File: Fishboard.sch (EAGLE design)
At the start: 21 parts, among them J3 B1, J4 B2, J5 B3, J7 B4, Q1 TIP120, Q2 TIP120, Q3 TIP120

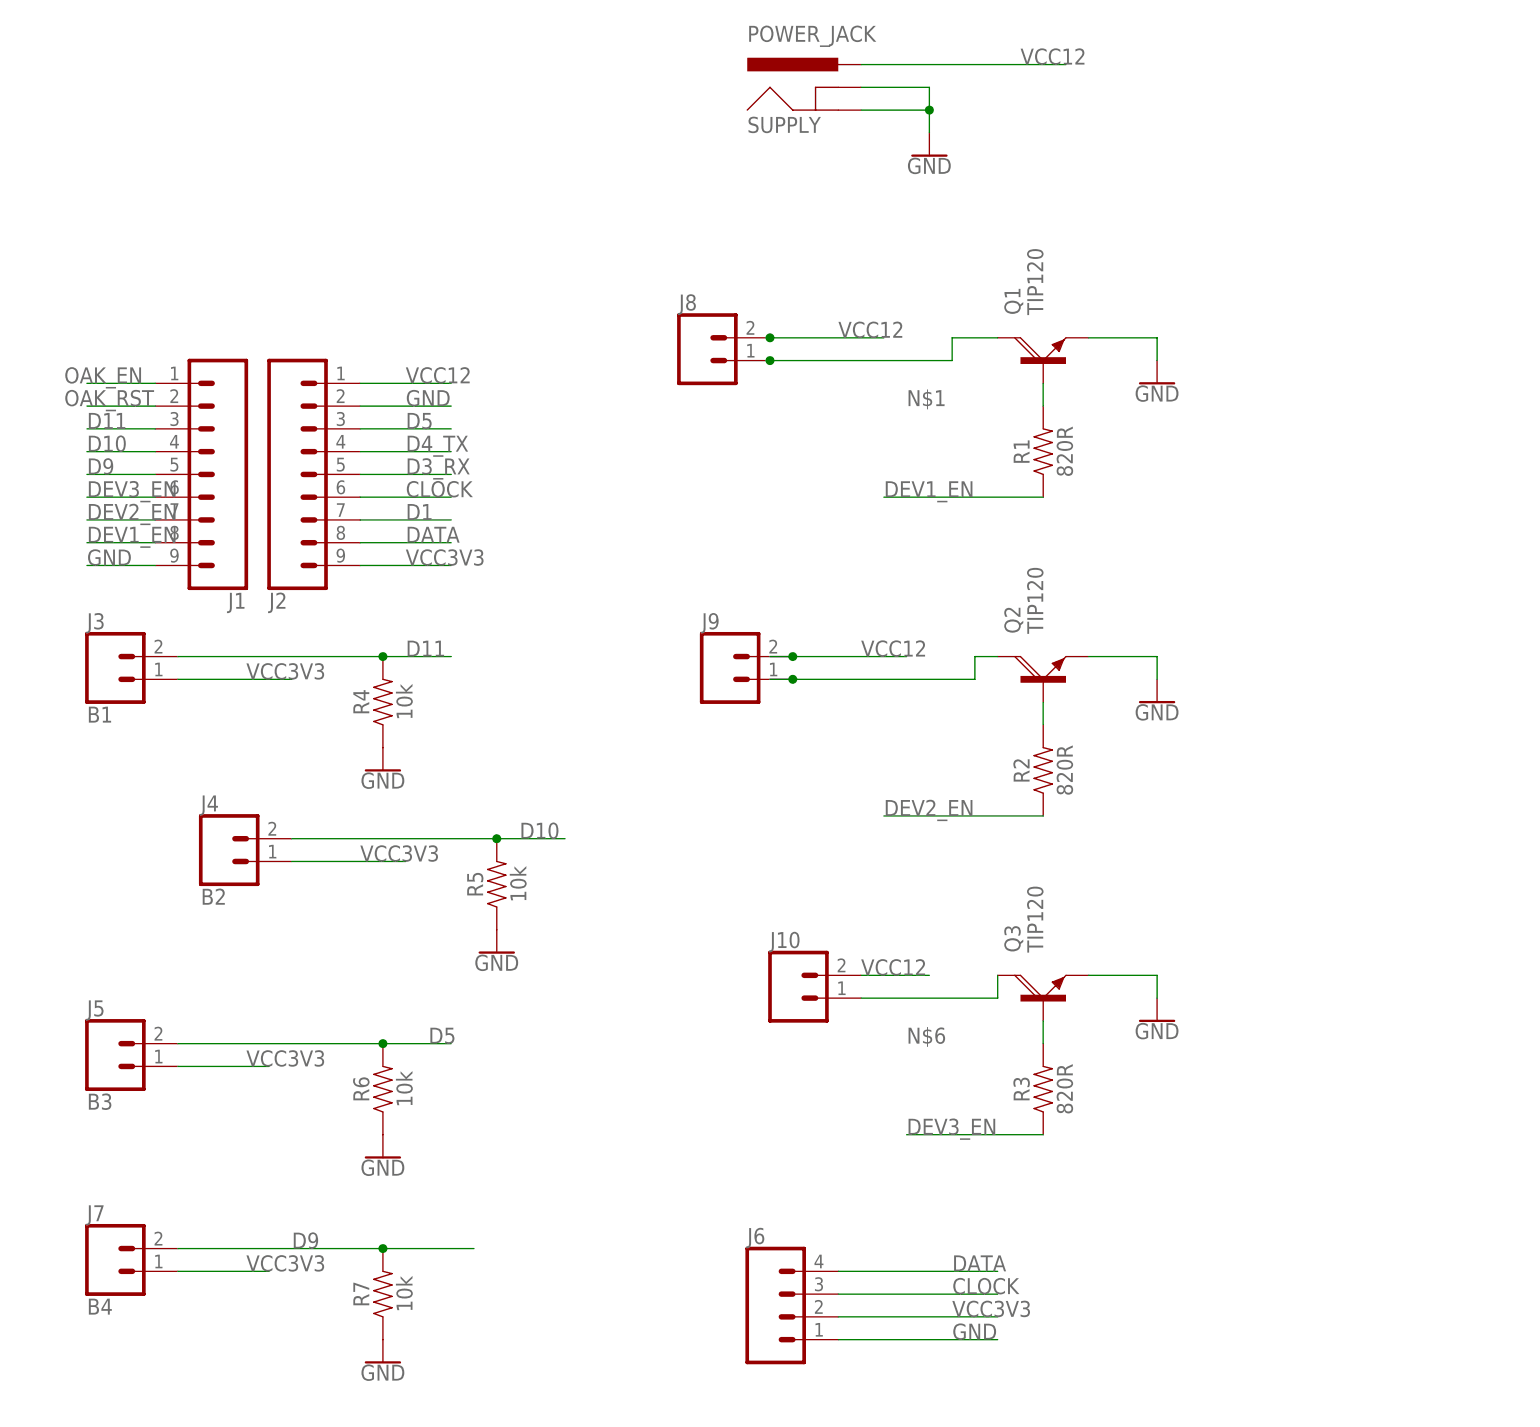
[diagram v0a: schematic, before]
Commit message: Reorganized schematics
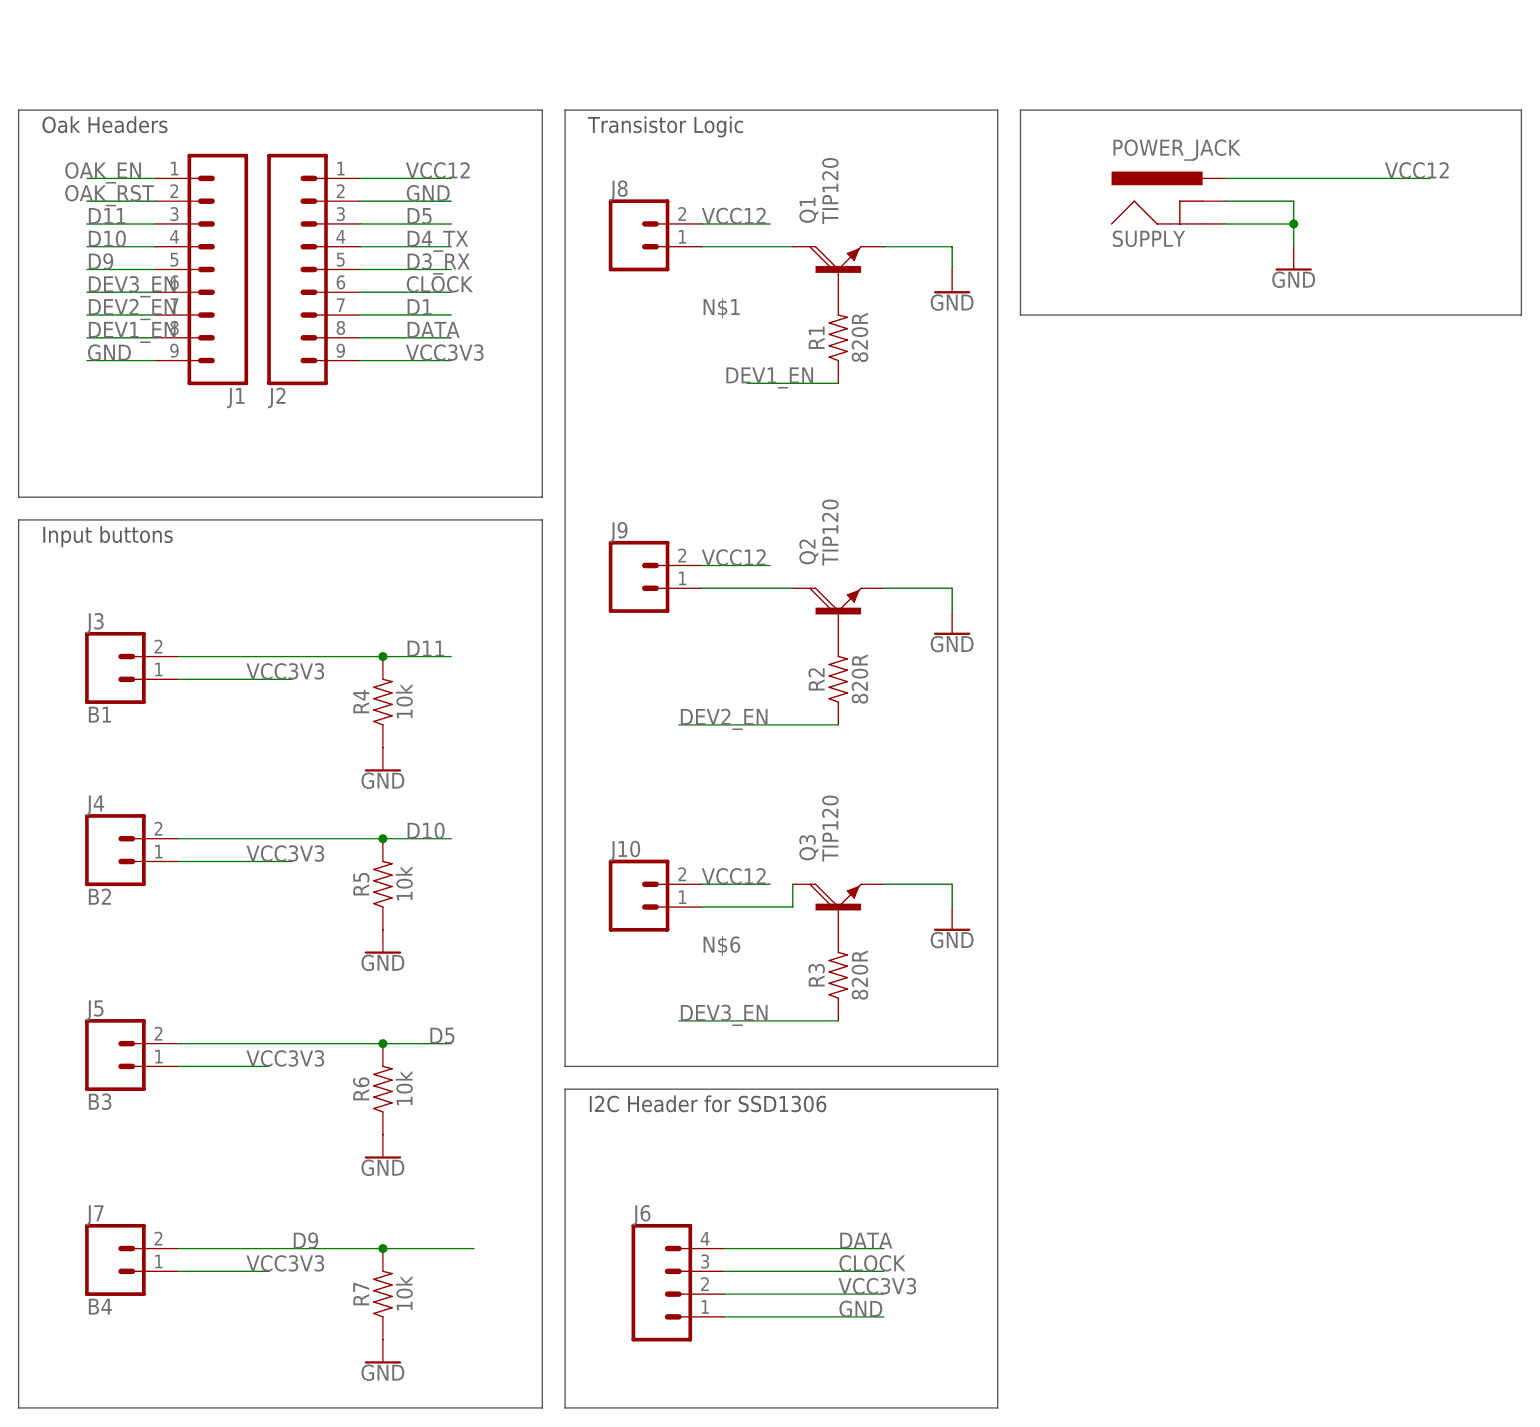
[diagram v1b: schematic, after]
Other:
- note added: "I2C Header for SSD1306"
- note added: "Input buttons"
- note added: "Oak Headers"
- note added: "Transistor Logic"
- moved on the sheet: J1, J10, J2, J4, J6, J8, J9, Q1, Q2, Q3, R1, R2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
